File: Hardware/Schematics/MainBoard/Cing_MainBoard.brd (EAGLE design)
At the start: 100 x 100 mm, 186 parts, among them IC1 L293D, IC2 LM2576S, IC3 FT232RL, IC4 BMP280, IC5 BME280, Q1 16mhz, Q2 BSS138, Q3 BSS138, Q4 BSS138, Q5 BSS138, Q6 NP2301AMR-G, Q7 NP2301AMR-G, T1 FS8205, T2 FS8205, U3 MPU-6050MPU6050, U4 CH330N

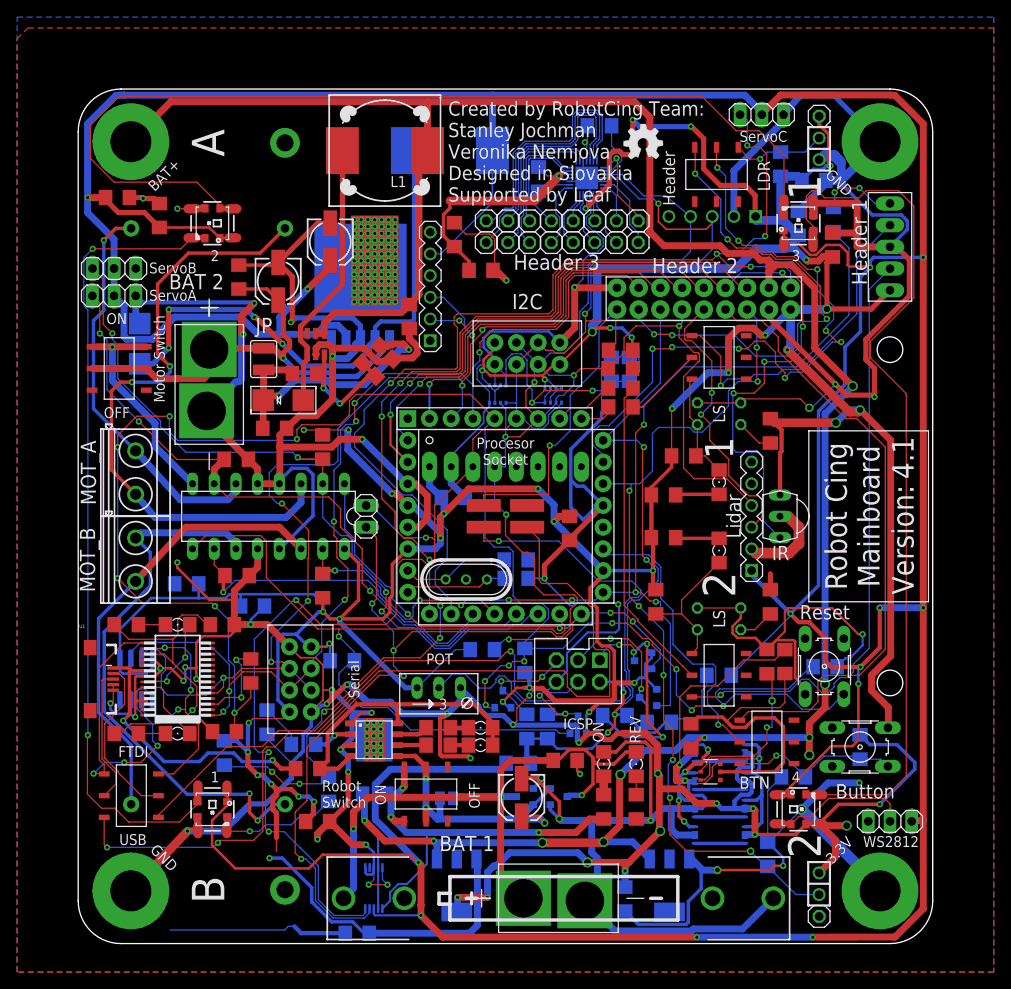
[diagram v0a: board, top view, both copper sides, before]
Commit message: small updates on Cing 4.1
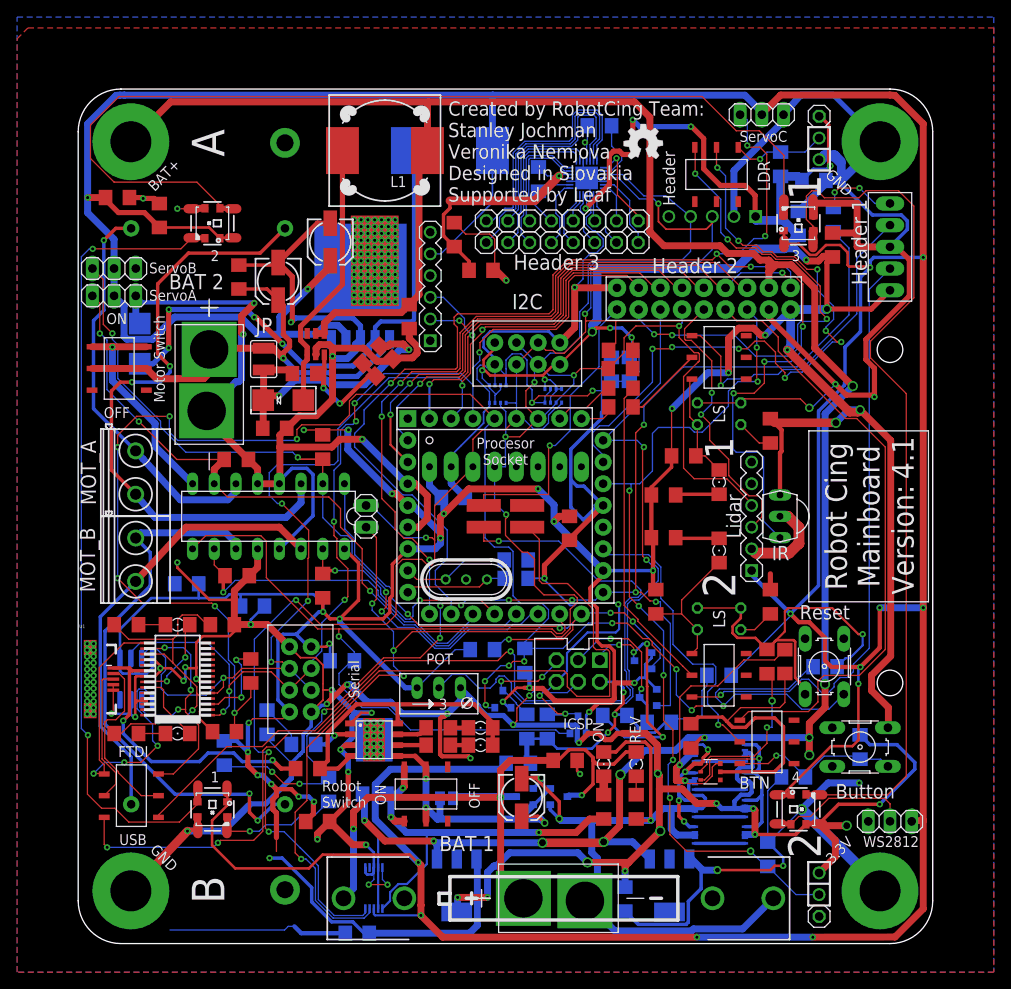
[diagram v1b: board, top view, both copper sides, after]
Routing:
- net VUSB: track 34.1 -> 35.0 mm
- net MOT_B-: track 65.2 -> 65.9 mm
- net +3V3: track 693.5 -> 694.1 mm
- net N$8: track 20.0 -> 20.6 mm
